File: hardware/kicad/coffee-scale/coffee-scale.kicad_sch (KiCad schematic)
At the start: 21 parts, among them J1 Conn_01x08, J3 Conn_01x02, Q1 DMG3415U, U1 ESP32-S3, U2 HX711, U3 MCP73832-5-OT, U4 AP2112/RT9080-3.3, X1MT1 JSTPH, X1MT2 JSTPH

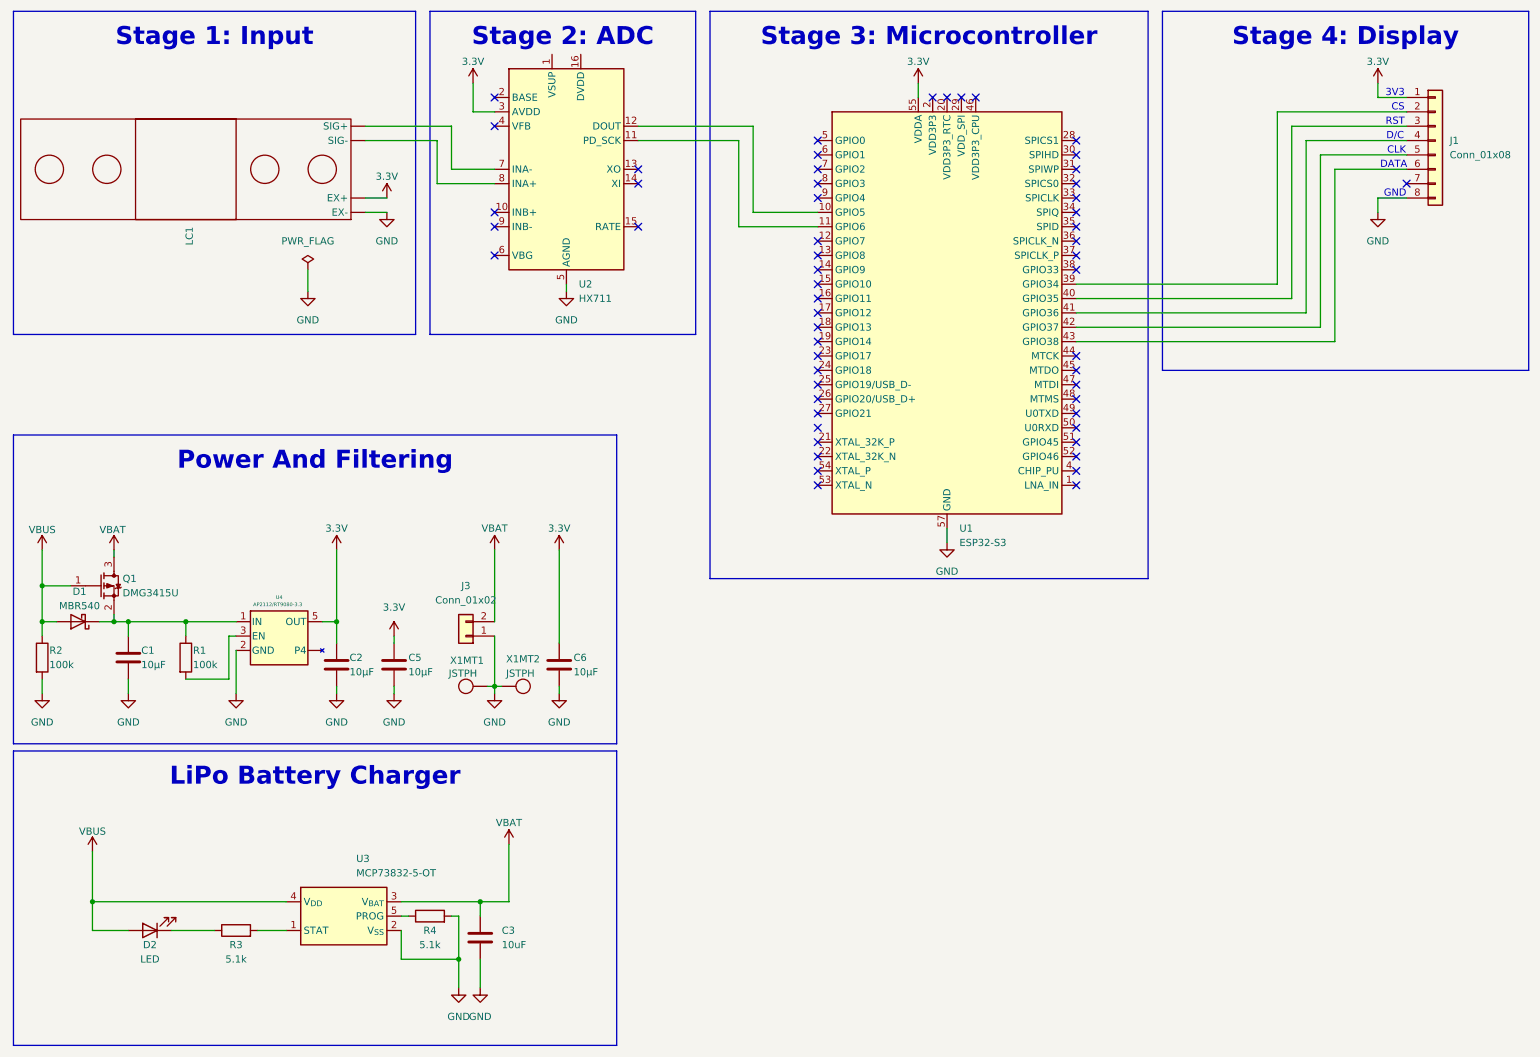
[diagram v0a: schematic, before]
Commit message: Update Stage 1 & Stage 2
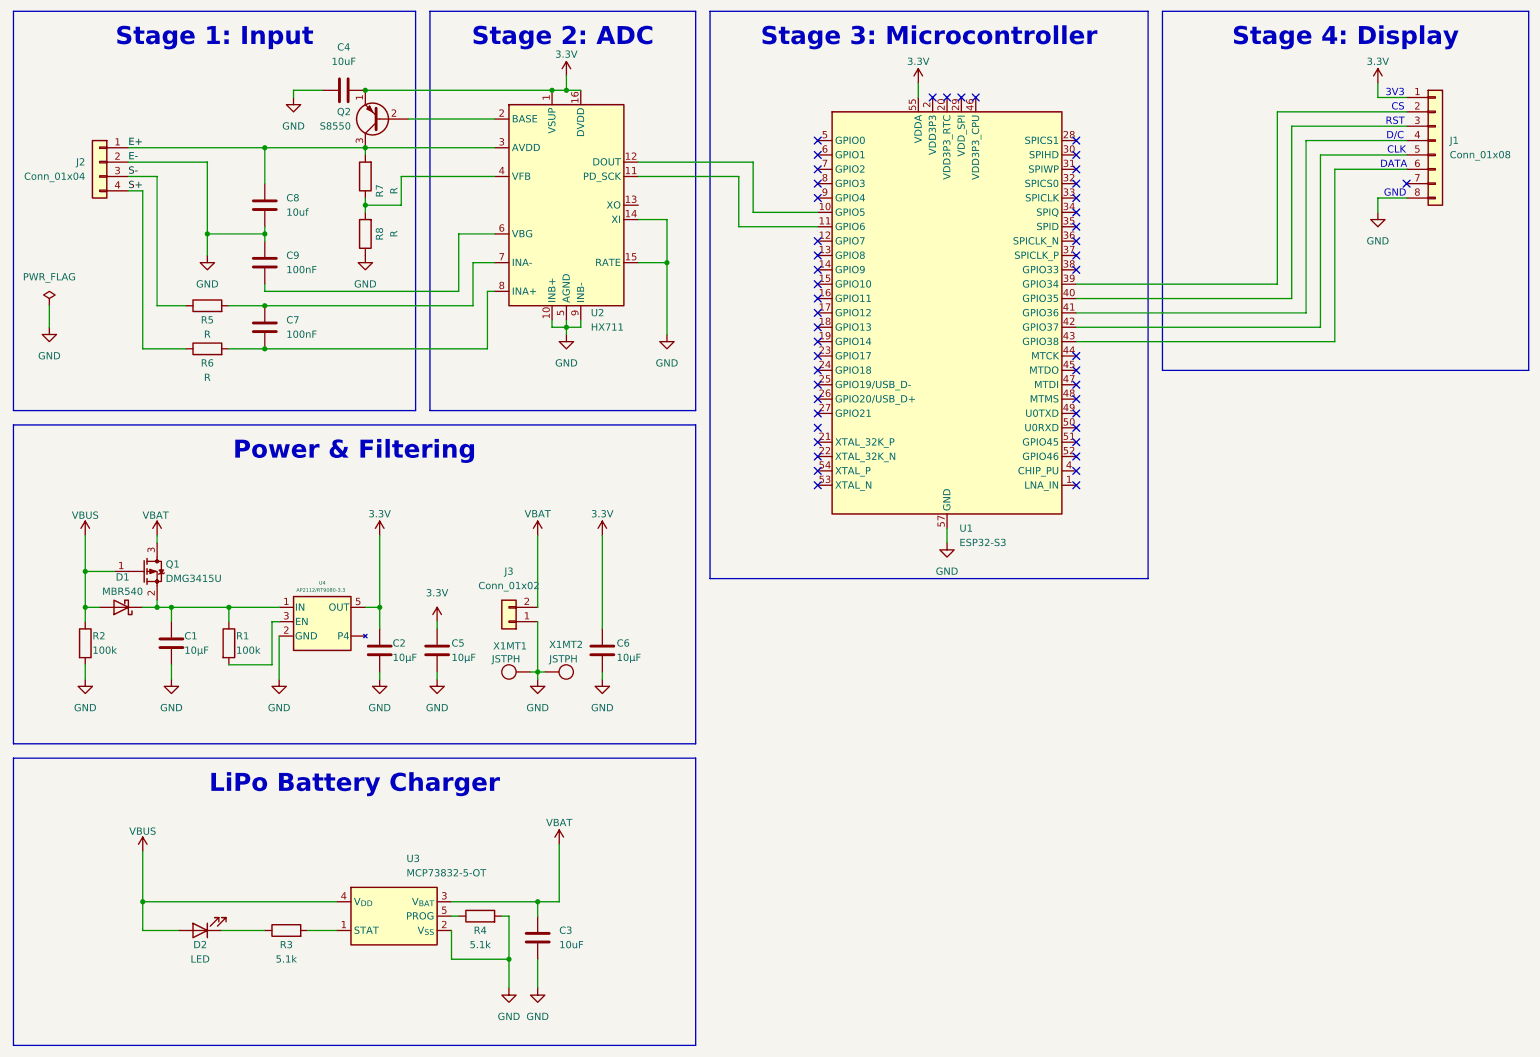
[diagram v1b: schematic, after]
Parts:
- removed LC1: ~, symbol Custom:4540
- added C4: 10uF, symbol Device:C
- added C7, C9: 100nF, symbol Device:C
- added C8: 10uf, symbol Device:C
- added J2: Conn_01x04, symbol Connector_Generic:Conn_01x04
- added Q2: S8550, Package_TO_SOT_THT:TO-92_Inline, symbol Transistor_BJT:S8550
- added R5, R6, R7, R8: R, symbol Device:R
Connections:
- net 3.3V: now also U2.1 (VSUP), U2.16 (DVDD), C4.1, Q2.1 (E); no longer U2.3 (AVDD)
- net GND: now also U2.10 (INB+), U2.14 (XI), U2.15 (RATE), U2.9 (INB-), C4.2, C8.2, C9.1, J2.2 (Pin_2), R8.1
- net at U2.7 (INA-): now also C7.1, R5.2
- net at U2.8 (INA+): now also C7.2, R6.2
- net at U2.2 (BASE): now also Q2.2 (B)
- net at U2.4 (VFB): now also R7.1, R8.2
- net at U2.6 (VBG): now also C9.2
- new net E+: C8.1, J2.1 (Pin_1), Q2.3 (C), R7.2, U2.3 (AVDD)
- new net S+: J2.4 (Pin_4), R6.1
- new net S-: J2.3 (Pin_3), R5.1
- no-connect marks 56 -> 48
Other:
- moved on the sheet: C1, C2, C3, C5, C6, D1, D2, J3, Q1, R1, R2, R3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
